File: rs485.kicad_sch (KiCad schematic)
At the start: 0 parts

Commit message: Corrected schematic and added new elements
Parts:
- added C13: 100nF/50V, Capacitors_Smd_0603:100nF_0603, symbol Capacitors_Smd0603:100n
- added D5, D7: SMAJ7.5CA, Diodes:SMAJ7.5CA_SMD_DO214AC, symbol Diodes:SMAJ7.5CA
- added D6: SMAJ18CA, Diodes:SMAJ18CA_SMD_DO214AC, symbol Diodes:SMAJ18CA
- added F3, F4: SN005-60, Smd_Ptc_Fuses:SN005-60, symbol Ptc_Smd_Fuses:SN005-60
- added R10, R9: CRCW120610R0FKEAHP, Resistor_Smd_1206:CRCW120610R0FKEAHP, symbol Resistors_Smd1206:CRCW120610R0FKEAHP
- added U10: ISL3172EIUZ, Communication_Interfaces:ISL3172EIUZ, symbol Communication_Interfaces:ISL3172EIUZ
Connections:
- new net: D5.2 (K), D6.1 (A), F3.1, R9.1
- new net: D6.2 (K), D7.1 (A), F4.1, R10.1
- new net: R10.2, U10.6 (A/Y)
- new net: R9.2, U10.7 (B/Z)
- new net GND: C13.2, D5.1 (A), D7.2 (K), U10.5 (GND)
- new net POWER_IN_3V3: C13.1, U10.8 (VCC)
- new net RS485_A: F4.2
- new net RS485_B: F3.2
- new net RS485_DIR: U10.2 (~RE), U10.3 (DE)
- new net RS485_RX: U10.1 (RO)
- new net RS485_TX: U10.4 (DI)

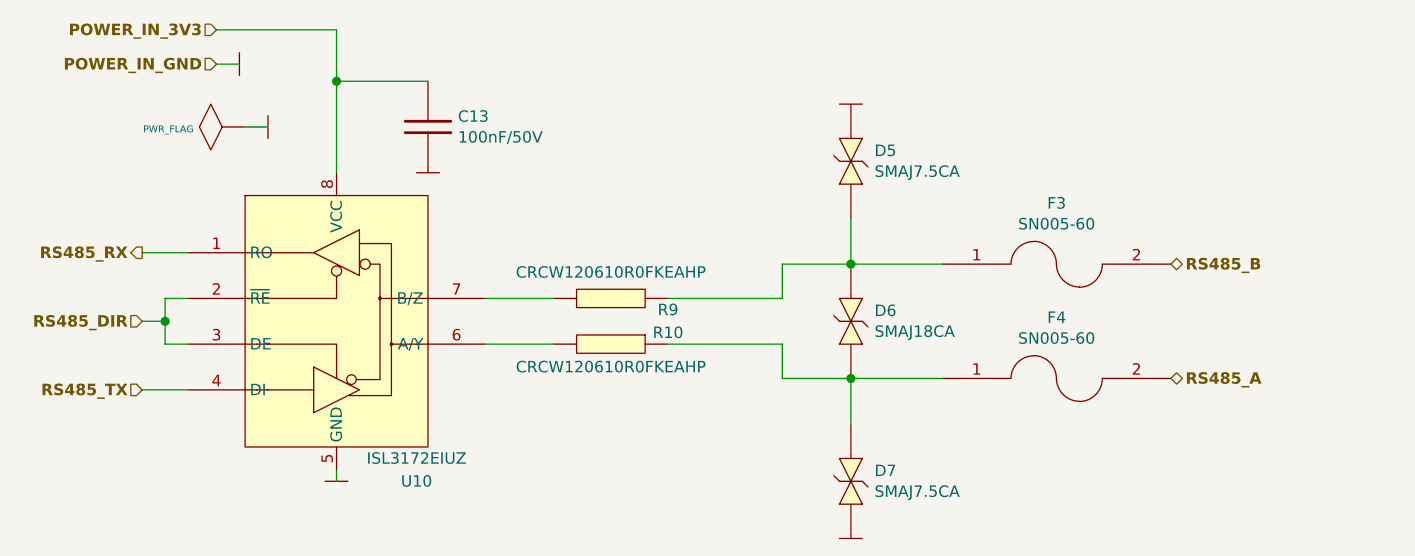
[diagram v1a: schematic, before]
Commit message: Finalized project
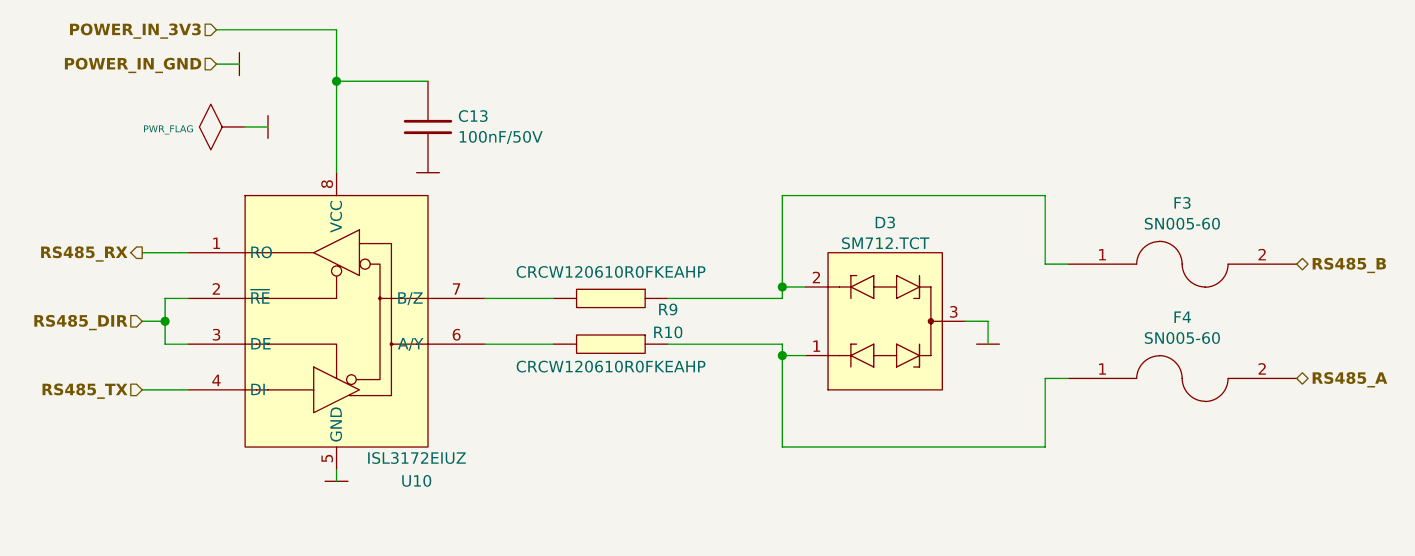
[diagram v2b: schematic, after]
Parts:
- removed D5, D7: SMAJ7.5CA, Diodes:SMAJ7.5CA_SMD_DO214AC, symbol Diodes:SMAJ7.5CA
- removed D6: SMAJ18CA, Diodes:SMAJ18CA_SMD_DO214AC, symbol Diodes:SMAJ18CA
- added D3: SM712.TCT, ESD_Protectors:SM712.TCT, symbol esd_protectors:SM712.TCT
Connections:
- net GND: now also D3.3 (GND)
- net at F3.1, R9.1: now also D3.2 (I/O2)
- net at F4.1, R10.1: now also D3.1 (I/O1)
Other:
- moved on the sheet: F3, F4
